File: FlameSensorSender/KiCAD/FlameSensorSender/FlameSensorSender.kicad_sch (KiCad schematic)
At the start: 36 parts, among them J1 SWD, J2 Sharp GP2Y1014AUOF, Q1 AO3400A, Q2 AO3400A, U1 STM32F103C6Tx, U2 Ai-Thinker-Ra-02, U3 MT3608, U4 MT3608

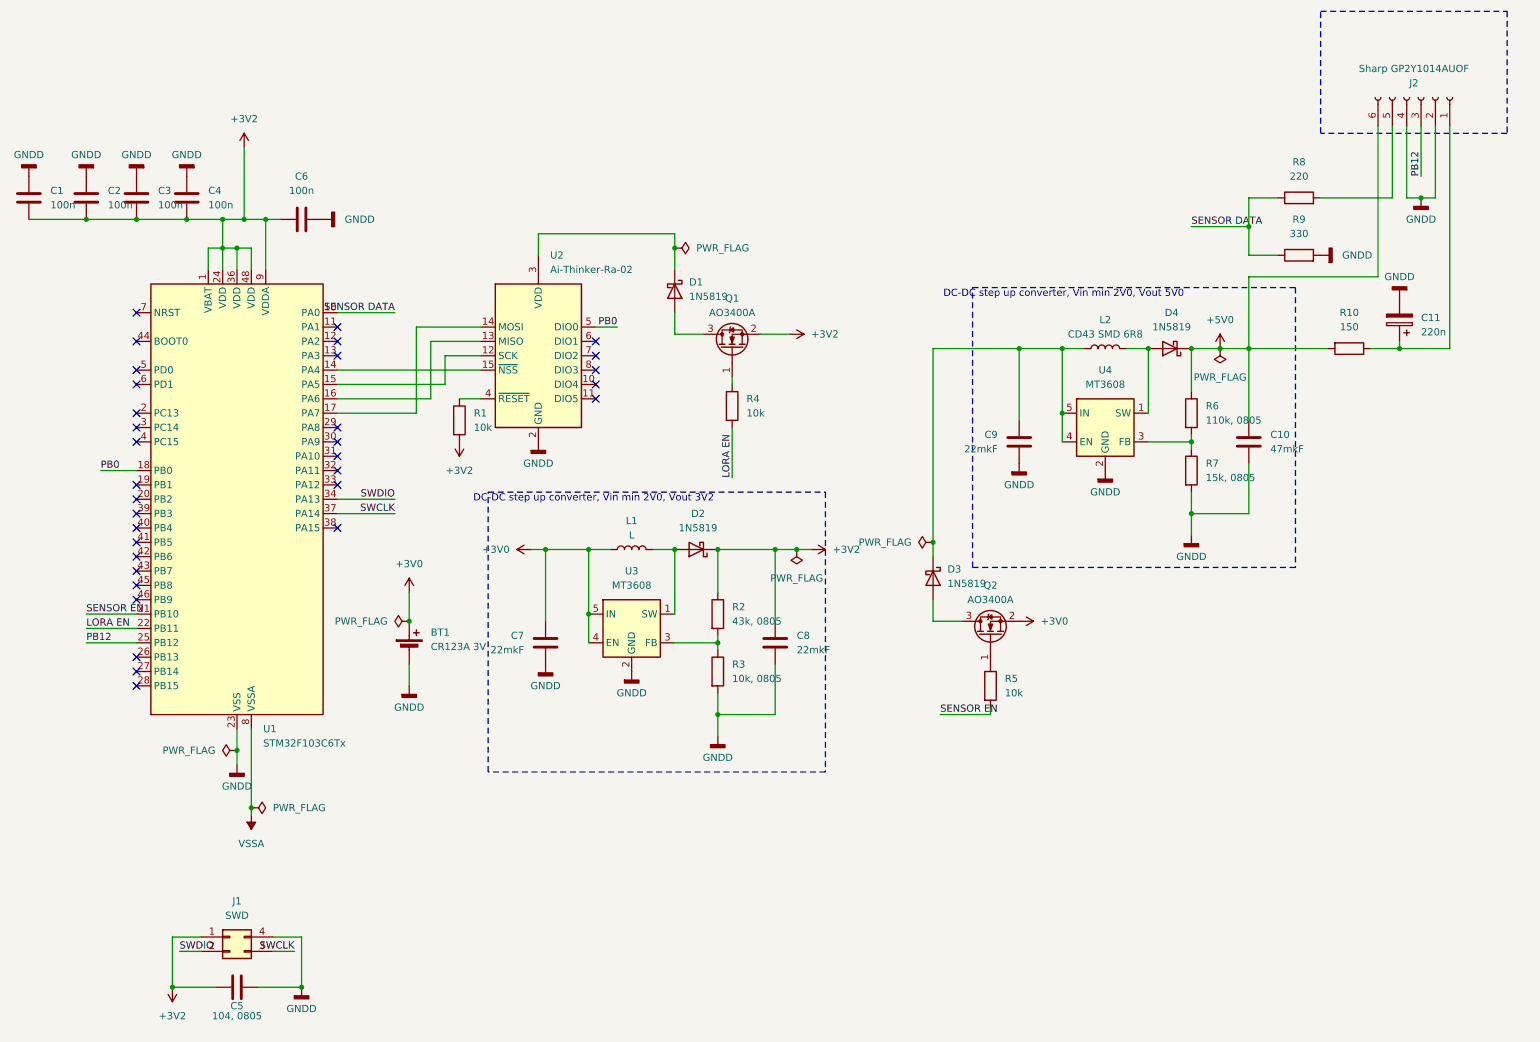
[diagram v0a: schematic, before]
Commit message: dev
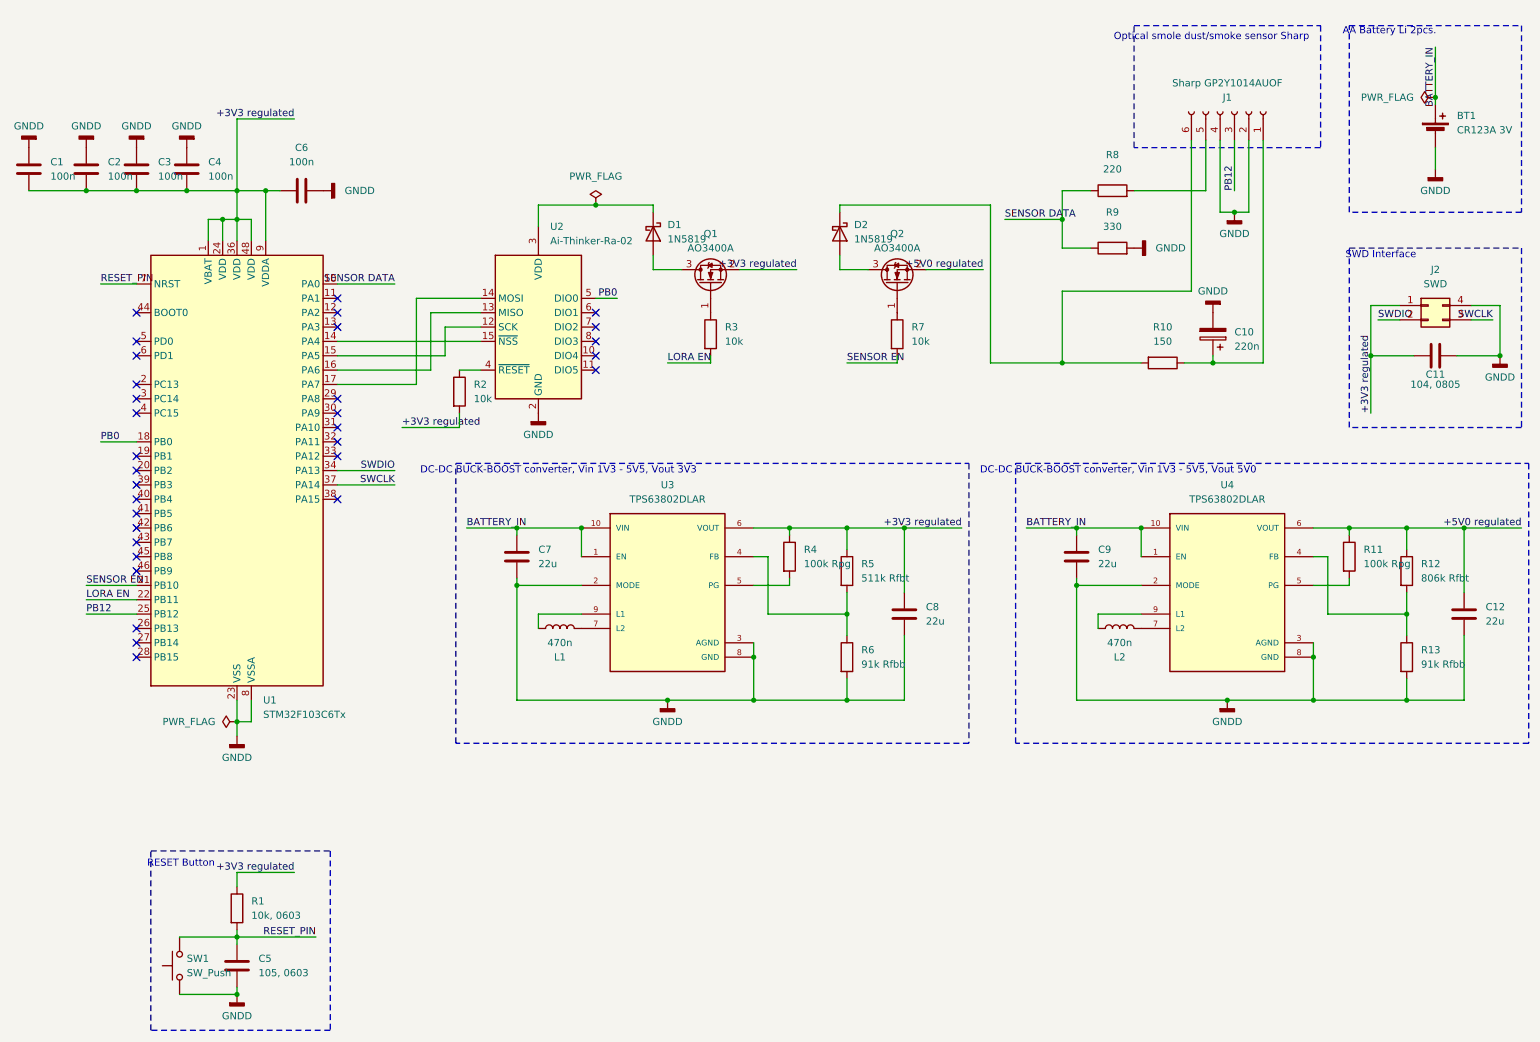
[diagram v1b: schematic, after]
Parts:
- removed C10: 47mkF, Capacitor_SMD:C_0805_2012Metric_Pad1.18x1.45mm_HandSolder, symbol Device:C
- removed D2, D4: 1N5819, Diode_SMD:D_0805_2012Metric_Pad1.15x1.40mm_HandSolder, symbol Diode:1N5819
- removed R2: 43k, 0805, Resistor_SMD:R_0805_2012Metric_Pad1.20x1.40mm_HandSolder, symbol Device:R
- removed R3: 10k, 0805, Resistor_SMD:R_0805_2012Metric_Pad1.20x1.40mm_HandSolder, symbol Device:R
- removed R7: 15k, 0805, Resistor_SMD:R_0805_2012Metric_Pad1.20x1.40mm_HandSolder, symbol Device:R
- removed U3, U4: MT3608, Package_TO_SOT_SMD:SOT-23-6, symbol Regulator_Switching:MT3608
- added C12: 22u, Capacitor_SMD:C_0603_1608Metric_Pad1.08x0.95mm_HandSolder, symbol Device:C
- added C5: 105, 0603, Capacitor_SMD:C_0603_1608Metric_Pad1.08x0.95mm_HandSolder, symbol Device:C
- added R1: 10k, 0603, Resistor_SMD:R_0603_1608Metric_Pad0.98x0.95mm_HandSolder, symbol Device:R
- added R11, R4: 100k Rpg, Resistor_SMD:R_0603_1608Metric_Pad0.98x0.95mm_HandSolder, symbol Device:R
- added R12: 806k Rfbt, Resistor_SMD:R_0603_1608Metric_Pad0.98x0.95mm_HandSolder, symbol Device:R
- added R13: 91k Rfbb, Resistor_SMD:R_0603_1608Metric_Pad0.98x0.95mm_HandSolder, symbol Device:R
- added R5: 511k Rfbt, Resistor_SMD:R_0603_1608Metric_Pad0.98x0.95mm_HandSolder, symbol Device:R
- added SW1: SW_Push, Button_Switch_THT:SW_PUSH_6mm_H4.3mm, symbol Switch:SW_Push
- added U3, U4: TPS63802DLAR, Footprints:VREG_TPS63802DLAR, symbol Custom_library:TPS63802DLAR
- C7, C8, C9: value 22mkF -> 22u; footprint Capacitor_SMD:C_0805_2012Metric_Pad1.18x1.45mm_HandSolder -> Capacitor_SMD:C_0603_1608Metric_Pad1.08x0.95mm_HandSolder
- L1: value L -> 470n; footprint Footprints:CD43 -> Inductor_SMD:L_Coilcraft_XxL4020
- L2: value CD43 SMD 6R8 -> 470n; footprint Footprints:CD43 -> Inductor_SMD:L_Coilcraft_XxL4020
- R6: value 110k, 0805 -> 91k Rfbb; footprint Resistor_SMD:R_0805_2012Metric_Pad1.20x1.40mm_HandSolder -> Resistor_SMD:R_0603_1608Metric_Pad0.98x0.95mm_HandSolder
- renumbered C11 to C10, C5 to C11, D3 to D2, J2 to J1, J1 to J2, R1 to R2, R4 to R3, R5 to R7
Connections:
- net VSSA is gone; now on net GNDD: U1.8 (VSSA)
- net GNDD: now also C7.2, C8.2, C9.2, R6.2, C12.2, C5.2, R13.2, SW1.1, U3.2 (MODE), U3.3 (AGND), U3.8 (GND), U4.2 (MODE), U4.3 (AGND), U4.8 (GND); no longer C7.1, C8.1, C9.1
- net at L1.2: now also U3.9 (L1)
- net at L2.2: now also U4.9 (L1)
- net RESET_PIN: now reaches U1.7 (NRST)
- net RESET_PIN: now also C5.1, R1.2, SW1.2
- removed net +3V0: BT1.1 (+), C7.2, L1.1, Q2.2 (S)
- net +3V2 renamed +3V3 regulated
- net +3V3 regulated: now also C8.1, R1.1, R4.1, R5.1, U3.6 (VOUT); no longer C8.2
- net +5V0: no longer names the net of J1.6 (Pin_6), R10.2
- net +5V0: now also D2.1 (K); no longer R6.1
- new net: R11.2, U4.5 (PG)
- new net: R5.2, R6.1, U3.4 (FB)
- new net: R4.2, U3.5 (PG)
- new net: R12.2, R13.1, U4.4 (FB)
- new net: L2.1, U4.7 (L2)
- new net: L1.1, U3.7 (L2)
- new net +5V0 regulated: C12.1, Q2.2 (S), R11.1, R12.1, U4.6 (VOUT)
- new net BATTERY_IN: BT1.1 (+), C7.1, C9.1, U3.1 (EN), U3.10 (VIN), U4.1 (EN), U4.10 (VIN)
- no-connect marks 33 -> 32
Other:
- note added: "AA Battery Li 2pcs."
- note added: "DC-DC BUCK-BOOST converter, Vin 1V3 - 5V5, Vout 3V3"
- note added: "DC-DC BUCK-BOOST converter, Vin 1V3 - 5V5, Vout 5V0"
- note added: "Optical smole dust/smoke sensor Sharp"
- note added: "RESET Button"
- note added: "SWD Interface"
- note removed: "DC-DC step up converter, Vin min 2V0, Vout 3V2"
- note removed: "DC-DC step up converter, Vin min 2V0, Vout 5V0"
- moved on the sheet: BT1, C1, C10, C11, C2, C3, C4, C6, D1, D2, J1, J2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
